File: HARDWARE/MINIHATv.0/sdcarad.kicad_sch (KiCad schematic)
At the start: 14 parts, among them J6 Micro_SD_Card_Det2

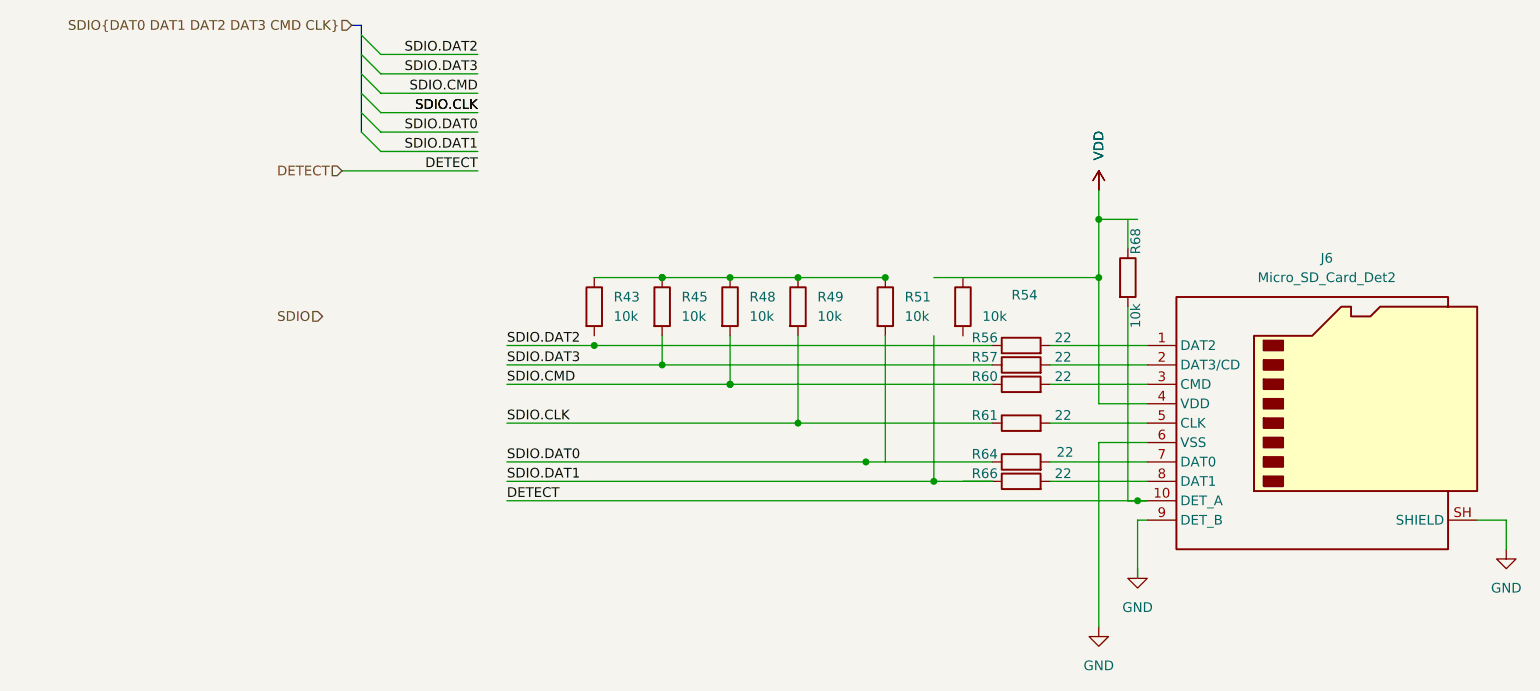
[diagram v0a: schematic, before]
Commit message: editorial changes
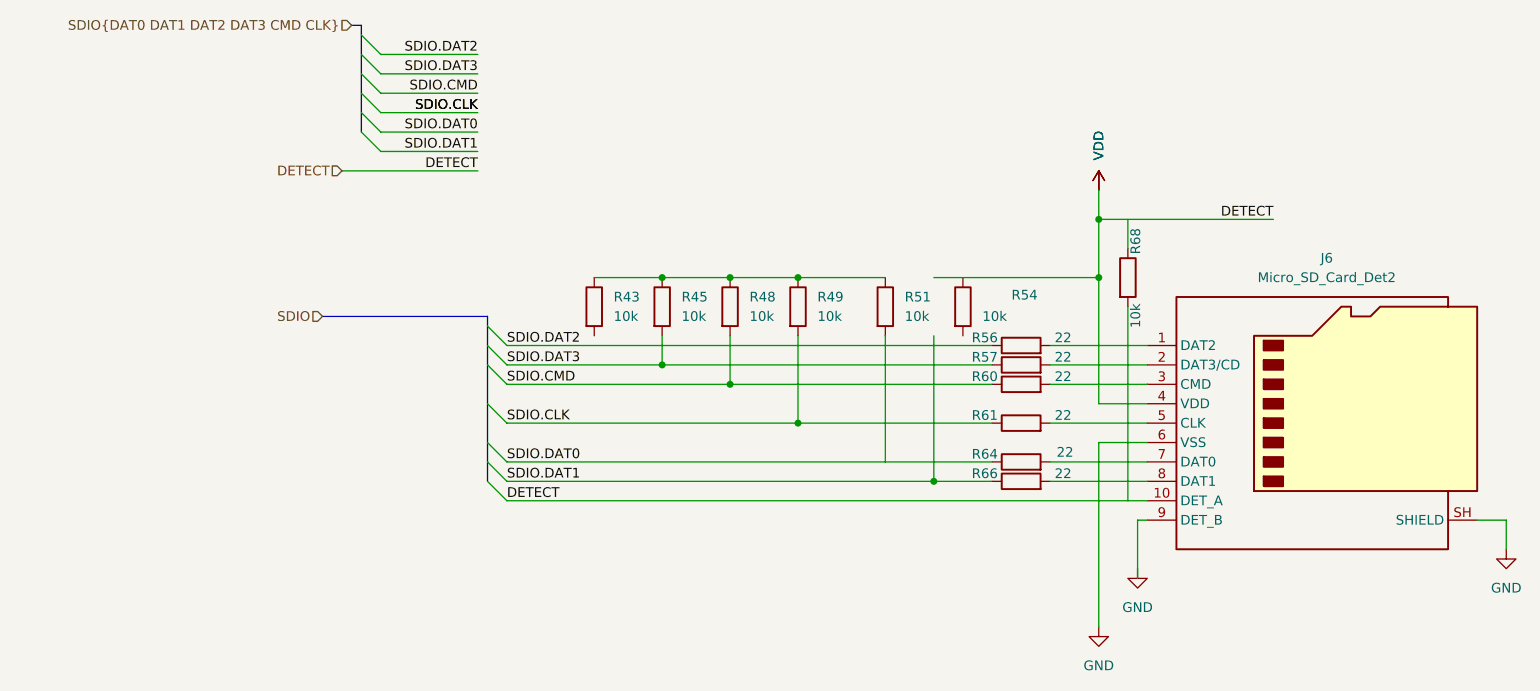
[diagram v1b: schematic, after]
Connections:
- net VDD: now also J6.10 (DET_A)
- net DETECT: no longer names the net of R68.2
- net DETECT: no longer J6.10 (DET_A)
